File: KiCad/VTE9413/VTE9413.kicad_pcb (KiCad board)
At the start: 2 copper layers, 73.7 x 48.3 mm, 24 parts, among them J1 Power, J2 Programmer, J3 Flowrate, J4 Flowrate, J5 Display, J6 Motorized valve, J7 Turbidity, J8 PH sensor, Q1 BD138, SW1 Switch, SW2 Reset, SW3 Mode, U1 L293D, U2 AMS1117-3.3, U3 ESP-12F

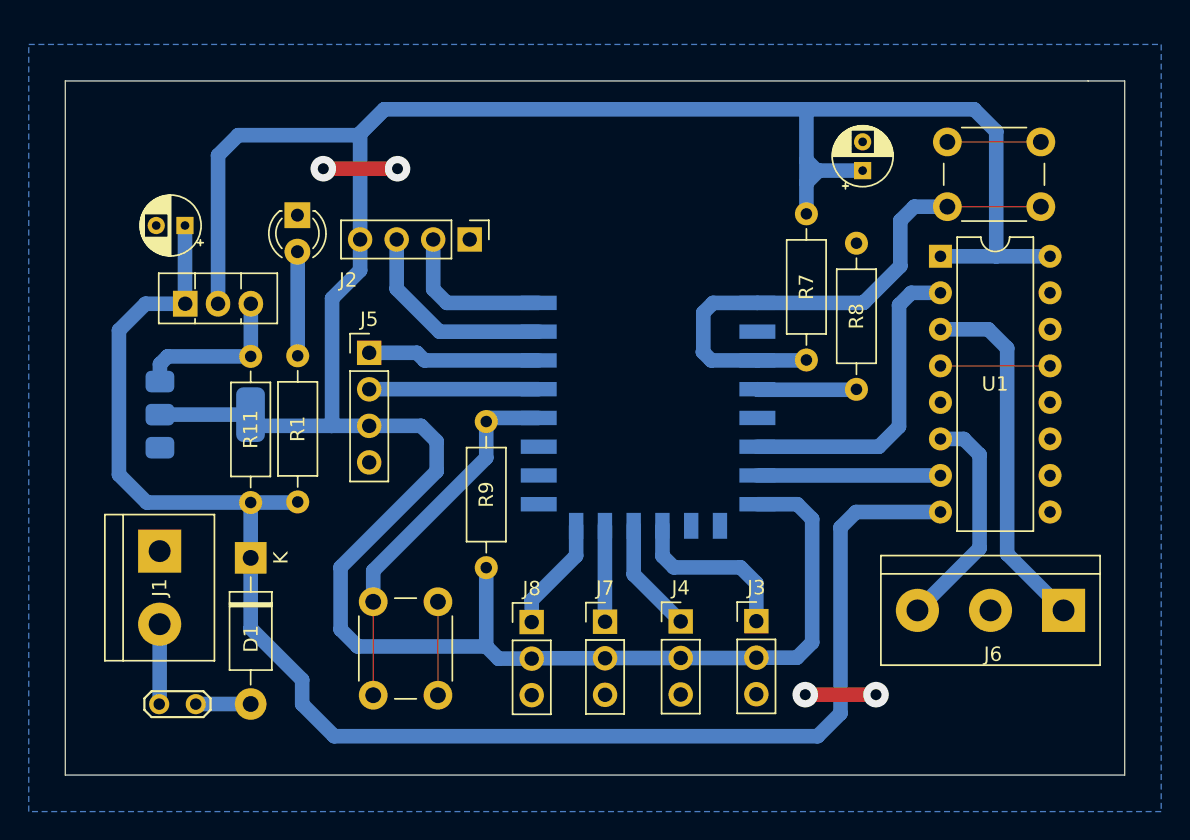
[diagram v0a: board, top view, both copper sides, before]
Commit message: Updates
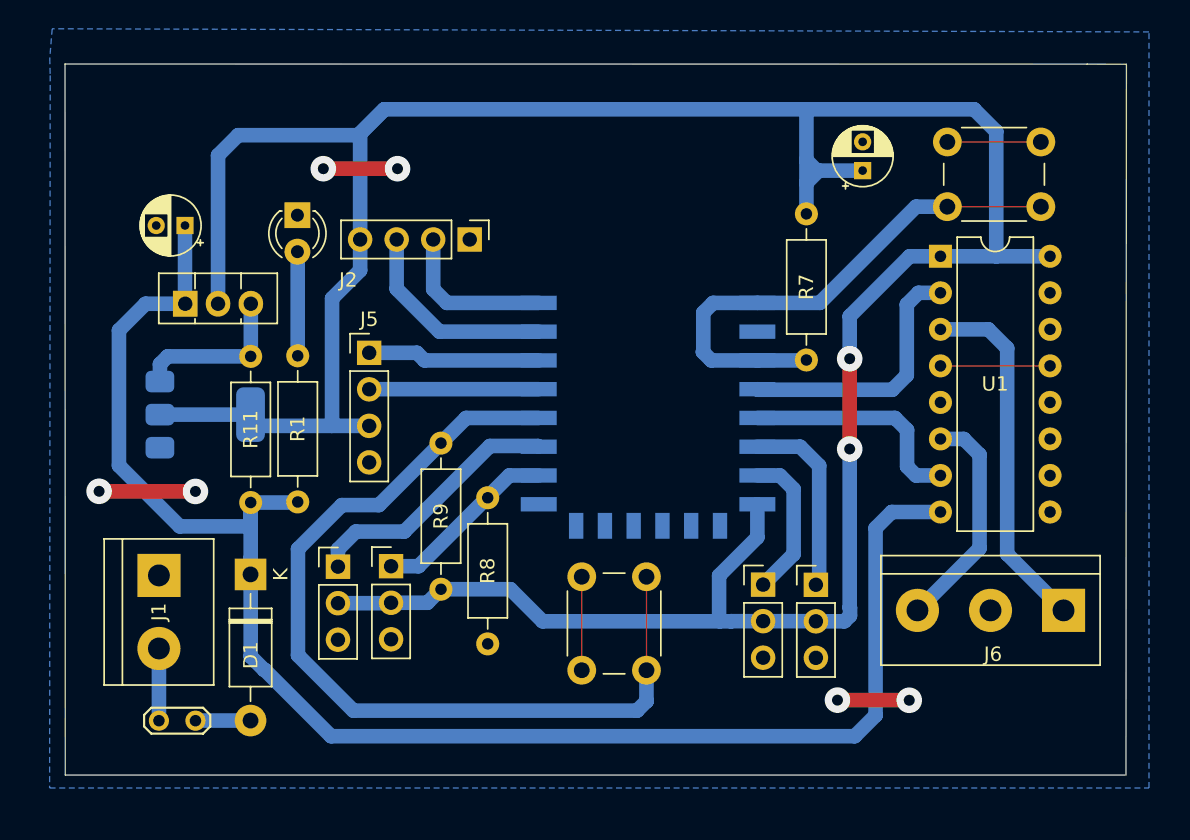
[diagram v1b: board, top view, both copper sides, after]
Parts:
- moved R8 26.7 mm to (100.5, 82.3), turned to -90 degrees
- moved J3 25.7 mm to (93.8, 87.1)
- moved J4 24.1 mm to (90.1, 87.1)
- moved SW3 20.7 mm to (111.5, 87.8), turned to -90 degrees
- moved J8 19.9 mm to (123.3, 88.4)
- moved J7 11.3 mm to (119.6, 88.4)
- moved R9 3.49 mm to (97.2, 88.7)
- moved J1 1.69 mm to (77.6, 87.7)
- moved SW1 1.15 mm to (77.6, 97.8)
- moved D1 1.15 mm to (84.0, 87.7)
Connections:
- R8 pad 1: Net-(U3-GPIO16) -> /flowrate1
- U3 pad 11: /flowrate1 -> unconnected-(U3-GPIO9-Pad11)
- U3 pad 12: /flowrate2 -> unconnected-(U3-GPIO10-Pad12)
- U3 pad 13: /turbidity -> unconnected-(U3-MOSI-Pad13)
- U3 pad 14: /ph -> unconnected-(U3-SCLK-Pad14)
- U3 pad 16: unconnected-(U3-GPIO15-Pad16) -> /flowrate1
- U3 pad 17: unconnected-(U3-GPIO2-Pad17) -> /flowrate2
- U3 pad 4: Net-(U3-GPIO16) -> /valve_pin1
- U3 pad 5: unconnected-(U3-GPIO14-Pad5) -> /valve_pin2
- U3 pad 6: /valve_pin1 -> /ph
- U3 pad 7: /valve_pin2 -> /turbidity
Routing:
- net Net-(SW3A-C): track 26.0 -> 62.7 mm
- net /flowrate2: track 8.00 -> 18.2 mm
- net Net-(U3-GPIO16): track 6.92 -> 0.00 mm
- net GND: track 30.7 -> 37.5 mm, vias 4 -> 6
- net /ph: track 7.97 -> 13.2 mm
- net /turbidity: track 6.67 -> 10.4 mm
- net /valve_pin1: track 22.1 -> 18.4 mm
- net /valve_pin2: track 12.7 -> 15.9 mm
- net +12V: track 108.9 -> 111.1 mm
- net +3.3V: track 207.4 -> 209.3 mm, vias 0 -> 2
- net Net-(SW2A-D): track 38.6 -> 36.7 mm
- net /flowrate1: track 12.1 -> 12.9 mm
- net Net-(J1-Pin_2): track 5.57 -> 5.02 mm
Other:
- board size 73.7 x 48.3 mm -> 73.8 x 49.5 mm
